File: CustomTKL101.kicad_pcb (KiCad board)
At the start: 2 copper layers, 422.3 x 131.8 mm, 223 parts, among them J1 USB4085-GF-A_REVA, SW1 SW_Push, U1 ATmega32U4-AU, Y1 16MHz

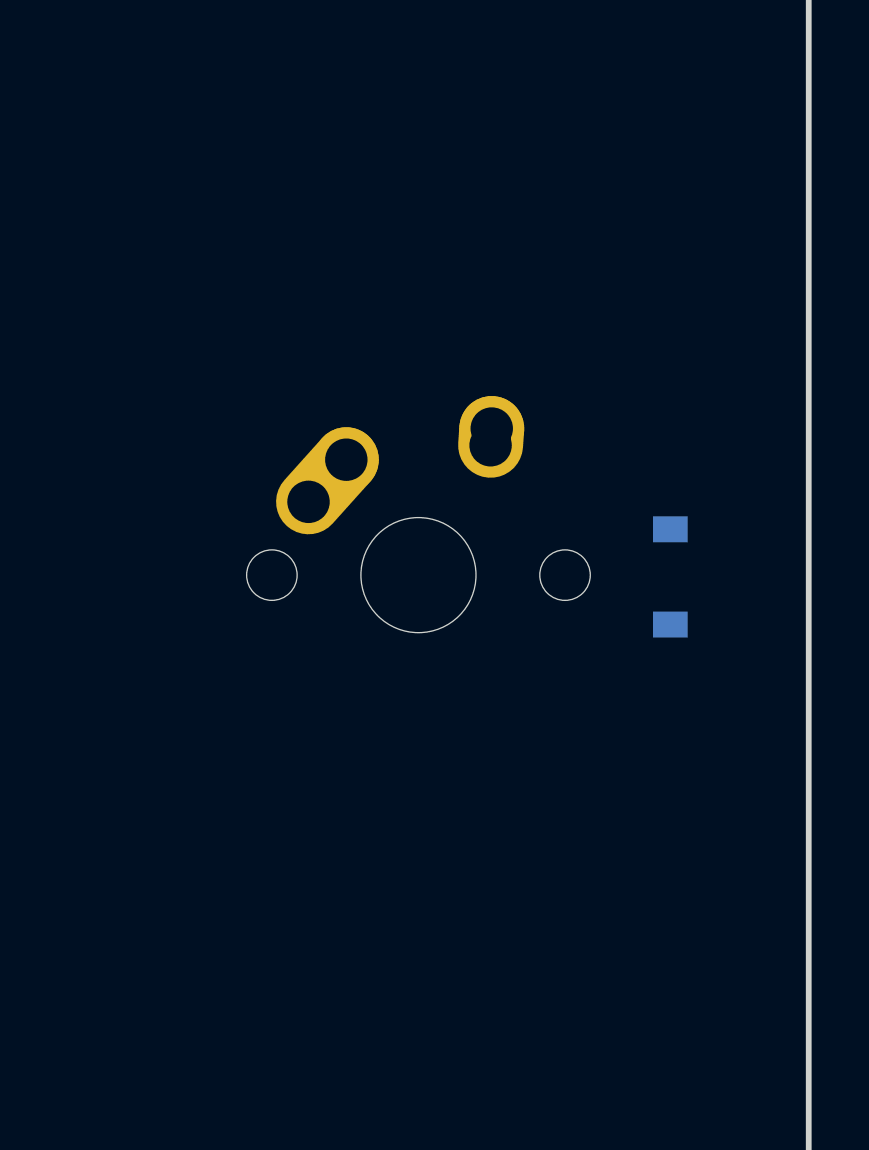
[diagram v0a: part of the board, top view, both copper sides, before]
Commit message: changed numenter footprint
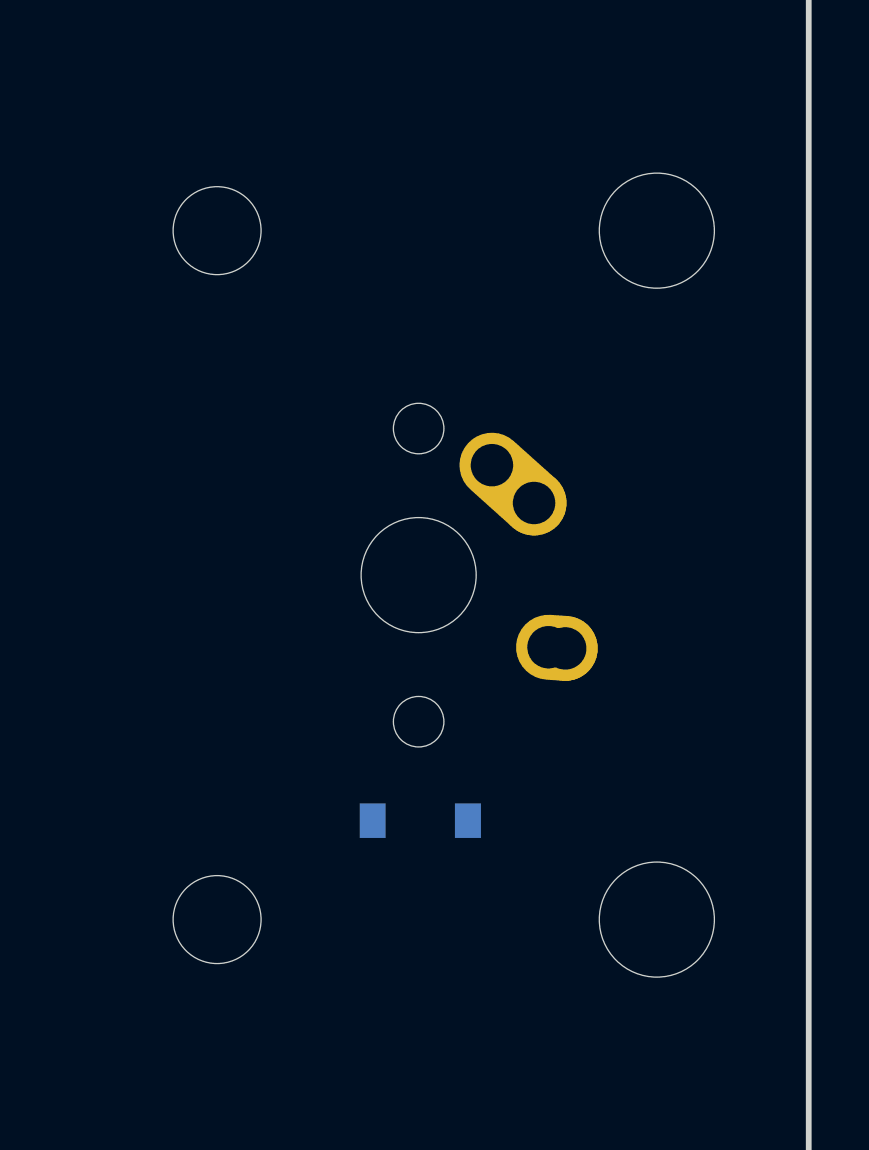
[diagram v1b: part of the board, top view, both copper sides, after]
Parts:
- K_87: footprint MX_Alps_Hybrid:MX-1U-NoLED -> MX_Alps_Hybrid:MX-2U-ReversedStabilizers-NoLED
- moved D_87 12.1 mm to (479.4, 187.1), turned to 0 degrees
- turned K_87 to 270 degrees
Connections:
- K_87 pad 1: col21 -> (no net)
- K_87 pad 2: Net-(D_87-Pad2) -> (no net)
